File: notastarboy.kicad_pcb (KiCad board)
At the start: 2 copper layers, 54.2 x 64.5 mm, 7 parts, among them J1 Conn_01x04_Pin, J2 Conn_01x08_Pin, SW1 SW_Push, SW2 SW_Push, U1 XIAO-ESP32-C3-SMD, U2 DHT11

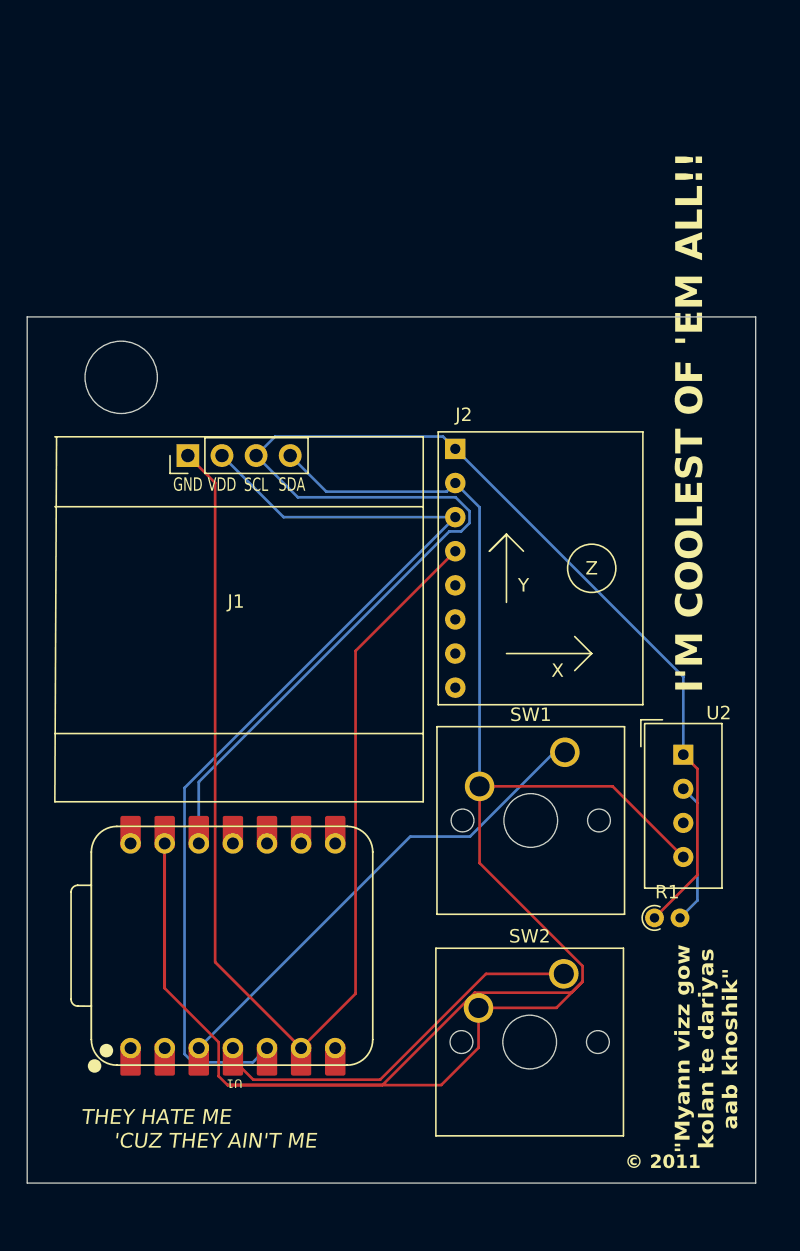
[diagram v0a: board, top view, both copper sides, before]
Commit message: final render and final pcb
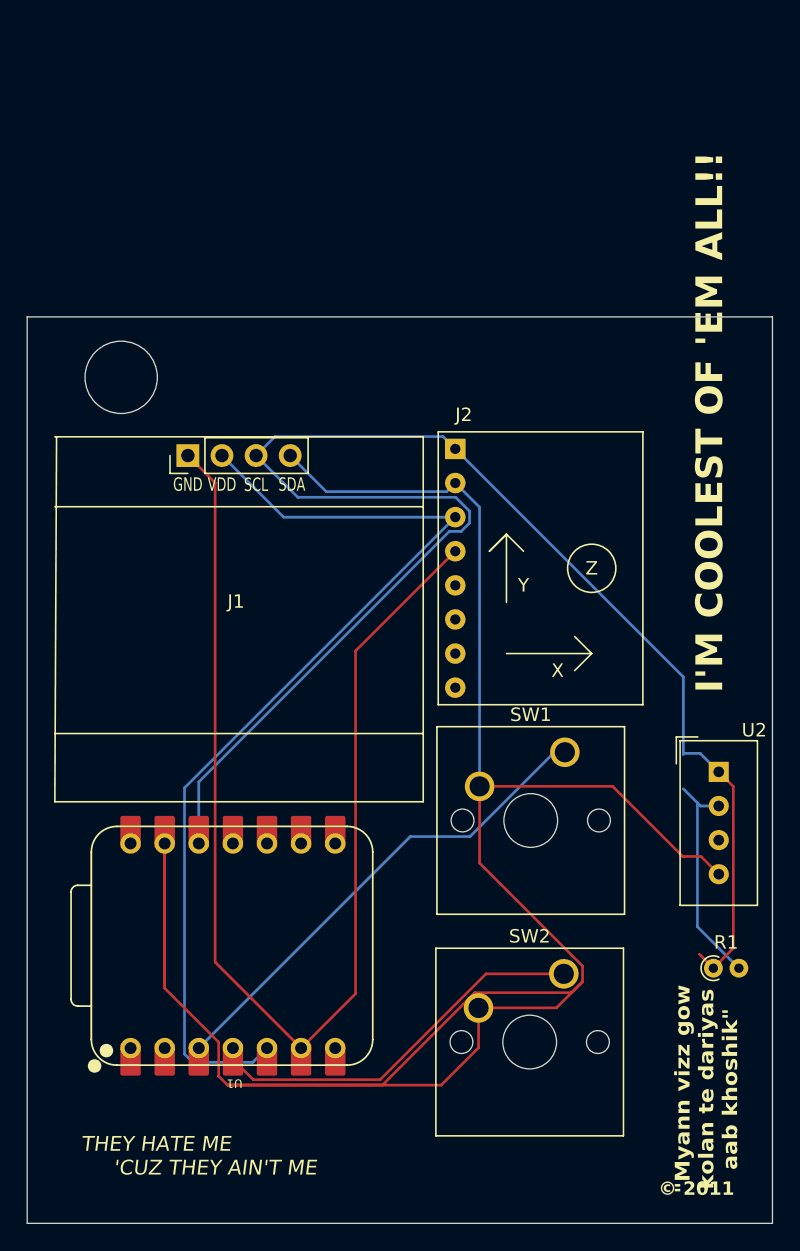
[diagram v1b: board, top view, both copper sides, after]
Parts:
- added G***: LOGO, graphics:omg, B.Cu at (108.0, 93.0)
- moved R1 5.77 mm to (129.6, 103.5)
- moved U2 2.93 mm to (130.0, 88.9)
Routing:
- net +3.3V: track 111.6 -> 118.0 mm
- net /DHT11 DATA: track 10.6 -> 16.8 mm
- net GND: track 164.6 -> 167.9 mm
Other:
- board size 54.2 x 64.5 mm -> 55.5 x 67.5 mm
